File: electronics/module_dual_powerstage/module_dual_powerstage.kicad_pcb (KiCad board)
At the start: 2 copper layers, 36.3 x 21.4 mm, 42 parts, among them J1 Conn_01x04, J2 Conn_01x04, Q1 60V4A, Q2 BC858B, Q3 BC847A, Q4 BC858B, Q5 BC847A, Q6 60V4A

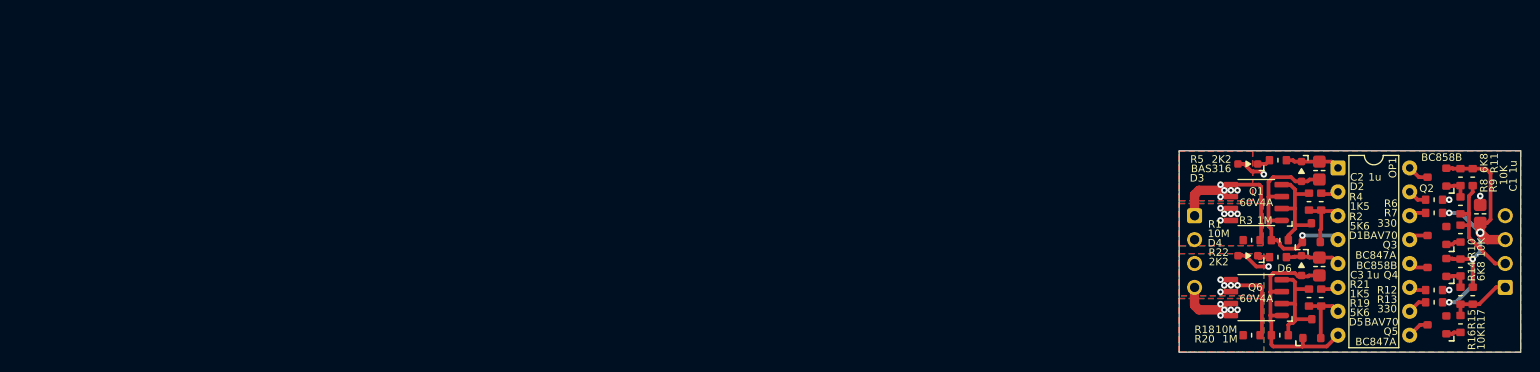
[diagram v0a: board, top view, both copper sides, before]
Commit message: added tiled version
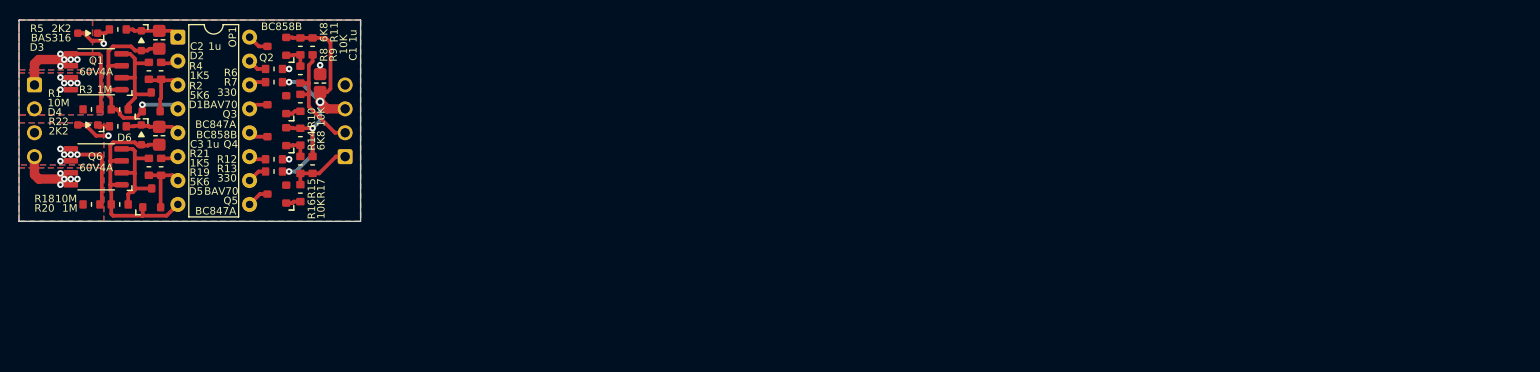
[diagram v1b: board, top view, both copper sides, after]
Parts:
- moved C1 124.1 mm to (62.0, 36.7)
- moved D2 124.1 mm to (43.0, 32.2)
- moved D5 124.1 mm to (44.1, 48.9)
- moved D6 124.1 mm to (43.0, 42.2)
- moved J2 124.1 mm to (64.7, 40.7)
- moved OP1 124.1 mm to (50.7, 40.7)
- moved R12 124.1 mm to (57.1, 44.8)
- moved R13 124.1 mm to (57.1, 46.1)
- moved R21 124.1 mm to (45.1, 45.6)
- moved R22 124.1 mm to (40.5, 41.3)
- moved R4 124.1 mm to (45.1, 35.4)
- moved R5 124.1 mm to (40.5, 31.0)
- moved R6 124.1 mm to (57.1, 35.2)
- moved R7 124.1 mm to (57.1, 36.6)
- moved D1 124.1 mm to (44.0, 38.7)
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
